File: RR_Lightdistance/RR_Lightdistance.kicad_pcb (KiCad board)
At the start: 2 copper layers, 34 x 40 mm, 62 parts, among them J1 Laser, Q1 2N7002, U1 MCP6002-xP, U2 MCP6002-xP, U3 ADS1115IDGS, U4 TP4056, U5 AP2112K-3.3, U6 MT3608, U7 MCP1700x-330xxTT, U8 ESP32-C3_SUPERMINI_TH

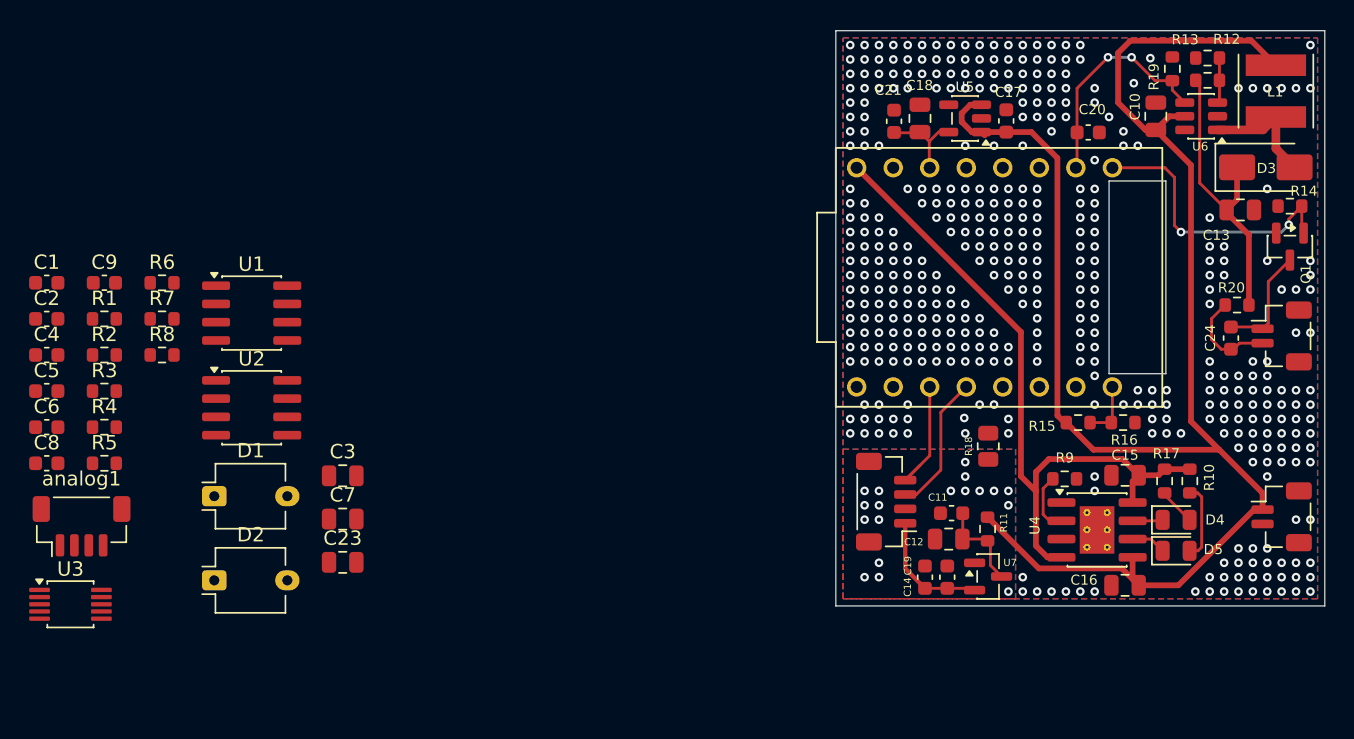
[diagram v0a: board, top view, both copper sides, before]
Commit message: mcp6004
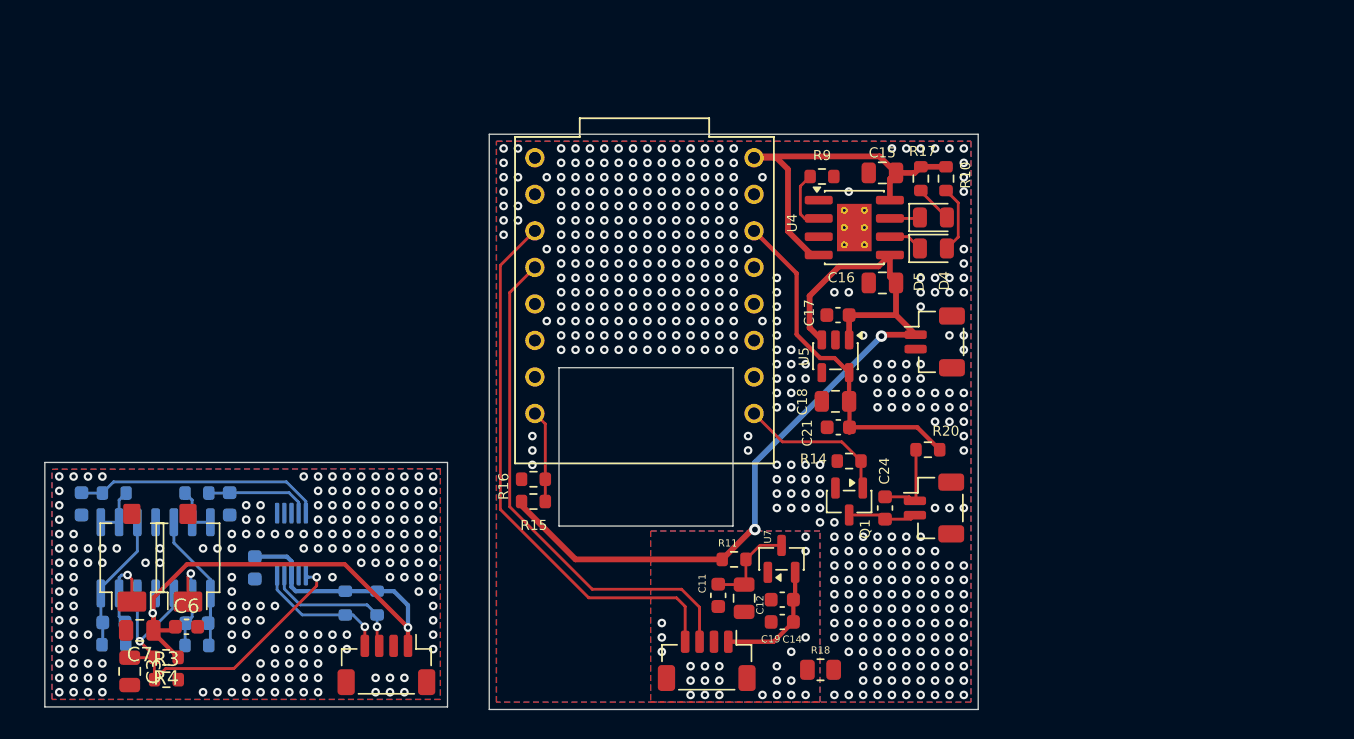
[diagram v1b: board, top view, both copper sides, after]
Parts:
- removed C10, C23: 10u, Capacitor_SMD:C_0805_2012Metric
- removed C13: 22u, Capacitor_SMD:C_0805_2012Metric
- removed C20, C5: 100n, Capacitor_SMD:C_0603_1608Metric
- removed D3: SS34, Diode_SMD:D_SMA
- removed L1: 22uH, Inductor_SMD:L_Taiyo-Yuden_MD-5050
- removed R12: 110k, Resistor_SMD:R_0603_1608Metric
- removed R13: 15k, Resistor_SMD:R_0603_1608Metric
- removed R19: 100k, Resistor_SMD:R_0603_1608Metric
- removed U1, U2: MCP6002-xP, Package_SO:SOIC-8_3.9x4.9mm_P1.27mm
- C1, C2, C4, C8, C9, R1, R2, R5, R6, R7, R8, U3: moved to B.Cu
- D1, D2: footprint OptoDevice:Osram_DIL2_4.3x4.65mm_P5.08mm -> OptoDevice:Osram_BPW34S-SMD
- R20: value 120R -> 47R
- U6: value MT3608 -> MCP6004; footprint Package_TO_SOT_SMD:SOT-23-6 -> Package_SO:SOIC-14_3.9x8.7mm_P1.27mm; moved to B.Cu
- moved U6 78.9 mm to (68.7, 80.7), turned to 90 degrees
- moved R16 41.2 mm to (95.0, 75.2), turned to 180 degrees
- moved R15 38.3 mm to (95.0, 76.7)
- moved Q1 35.4 mm to (116.9, 76.7)
- moved R14 35.4 mm to (116.9, 73.9)
- moved J3 27.0 mm to (122.9, 65.6)
- moved R10 27.0 mm to (123.7, 54.3)
- moved R17 27.0 mm to (121.9, 54.3)
- moved J1 27.0 mm to (122.8, 77.2)
- moved C15 27.0 mm to (119.2, 53.9)
- moved C16 27.0 mm to (119.2, 61.5)
- moved D4 27.0 mm to (122.8, 57.0)
- moved D5 27.0 mm to (122.8, 59.1)
- moved R9 27.0 mm to (115.0, 54.1)
- moved U4 27.0 mm to (117.3, 57.7)
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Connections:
- C1 pad 1: Net-(U2A-+) -> Net-(U6D-+)
- C2 pad 1: Net-(U2B-+) -> Net-(U6C-+)
- C24 pad 1: Net-(J1-Pin_2) -> Net-(J1-Pin_1)
- J1 pad 1: /Digital/LASER_EN -> Net-(J1-Pin_1)
- J1 pad 2: Net-(J1-Pin_2) -> /Digital/LASER_EN
- R1 pad 1: Net-(U2A-+) -> Net-(U6D-+)
- R2 pad 1: Net-(U2B-+) -> Net-(U6C-+)
- R20 pad 1: /Laser/5V_LASER -> /Digital/3V3_DIG
- R20 pad 2: Net-(J1-Pin_2) -> Net-(J1-Pin_1)
- R5 pad 1: Net-(U2A--) -> Net-(U6D--)
- R6 pad 1: Net-(U2B--) -> Net-(U6C--)
- U6 pad 1: Net-(D3-A) -> Net-(U6D-+)
- U6 pad 2: /Digital/GND_DIG -> Net-(D1-K)
- U6 pad 3: Net-(U6-FB) -> /Analog/Vbias
- U6 pad 4: /Digital/BOOST_EN -> /Analog/3V3_ANA
- U6 pad 5: /Power/VBAT -> /Analog/Vbias
- U6 pad 6: unconnected-(U6-NC-Pad6) -> Net-(D2-K)
- U8 pad 1: /Digital/BOOST_EN -> unconnected-(U8-GPIO1-Pad1)
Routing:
- net /Power/VBAT: track 116.8 -> 59.9 mm, vias 0 -> 2
- net /Analog/3V3_ANA: track 8.97 -> 55.2 mm, vias 0 -> 2
- net /Analog/SCL: track 8.64 -> 48.0 mm, vias 0 -> 1
- net /Analog/SDA: track 9.69 -> 46.2 mm, vias 0 -> 1
- net /Analog/Vbias: track 0.00 -> 27.9 mm, vias 0 -> 2
- net /Digital/5V_IN: track 48.7 -> 25.9 mm
- net /Laser/5V_LASER: track 20.4 -> 0.00 mm
- net /Digital/3V3_DIG: track 5.48 -> 24.3 mm
- net Net-(U3-AIN1): track 0.00 -> 17.3 mm
- net /Digital/BOOST_EN: track 15.6 -> 0.00 mm, vias 2 -> 0
- net Net-(U6D-+): track 0.00 -> 11.8 mm
- net Net-(U6C-+): track 0.00 -> 9.65 mm
- net Net-(Q1-G): track 19.9 -> 10.7 mm, vias 2 -> 0
- net Net-(D3-A): track 8.47 -> 0.00 mm
- net Net-(D2-K): track 0.00 -> 7.50 mm, vias 0 -> 1
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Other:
- board size 34 x 40 mm -> 64.9 x 40 mm
